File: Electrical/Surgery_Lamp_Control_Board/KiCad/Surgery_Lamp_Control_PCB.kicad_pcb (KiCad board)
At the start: 2 copper layers, 90 x 60 mm, 44 parts, among them J1 OSTVN05A150, J2 Headlamp, J3 Joint 1 Encoder, J4 Joint 2 Encoder, J5 joint2, J6 joint3, J7 joint4, J8 Stepper, Q1 BSS138, Q2 BSS138, Q3 BSS138, Q4 BSS138, Q5 BSS138, Q6 BSS138, U1 MAX485E, U2 PCA9685PW

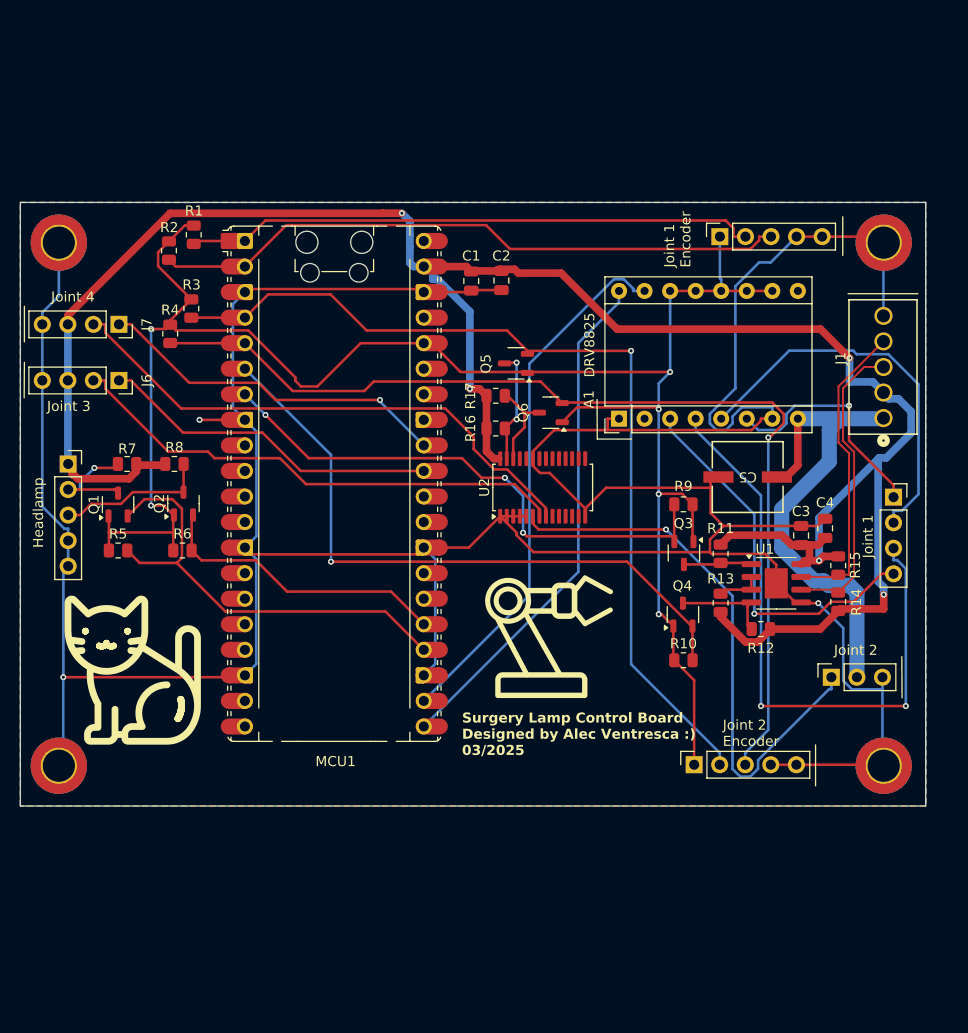
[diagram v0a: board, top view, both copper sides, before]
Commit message: Update Surgery Lamp Control PCB files
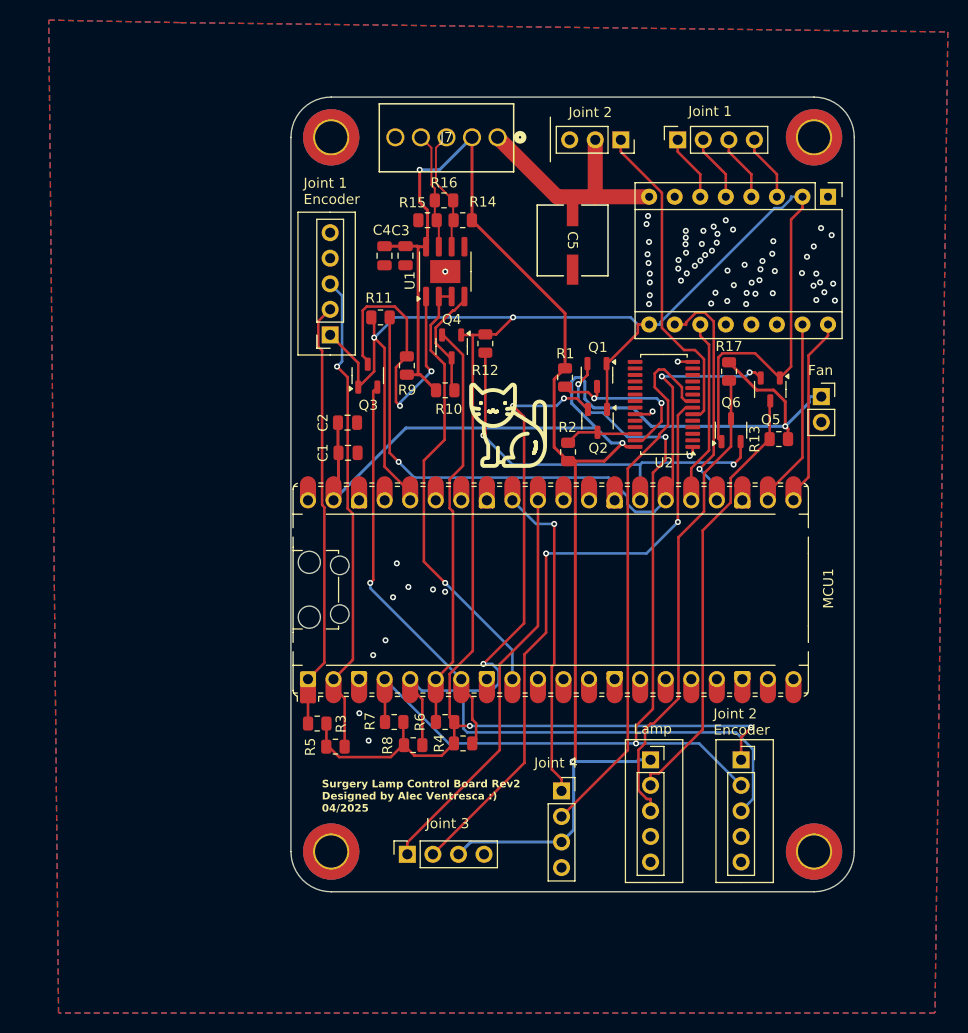
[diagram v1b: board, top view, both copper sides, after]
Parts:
- added J9: Fan, Connector_PinSocket_2.54mm:PinSocket_1x02_P2.54mm_Vertical, F.Cu at (176.0, 94.0)
- A1: value Pololu_Breakout_DRV8825 -> TMC2209 Stepper Driver
- J1: value OSTVN05A150 -> joint2; footprint Alec_lib:CONN5_516x256_OST -> Connector_PinSocket_2.54mm:PinSocket_1x03_P2.54mm_Vertical
- J2: value Headlamp -> joint3; footprint Connector_PinSocket_2.54mm:PinSocket_1x05_P2.54mm_Vertical -> Connector_PinSocket_2.54mm:PinSocket_1x04_P2.54mm_Vertical
- J3: value Joint 1 Encoder -> joint4; footprint Connector_PinSocket_2.54mm:PinSocket_1x05_P2.54mm_Vertical -> Connector_PinSocket_2.54mm:PinSocket_1x04_P2.54mm_Vertical
- J4: value Joint 2 Encoder -> Headlamp
- J5: value joint2 -> Joint 1 Encoder; footprint Connector_PinSocket_2.54mm:PinSocket_1x03_P2.54mm_Vertical -> Connector_PinSocket_2.54mm:PinSocket_1x05_P2.54mm_Vertical
- J6: value joint3 -> Joint 2 Encoder; footprint Connector_PinSocket_2.54mm:PinSocket_1x04_P2.54mm_Vertical -> Connector_PinSocket_2.54mm:PinSocket_1x05_P2.54mm_Vertical
- J7: value joint4 -> OSTVN05A150; footprint Connector_PinSocket_2.54mm:PinSocket_1x04_P2.54mm_Vertical -> Alec_lib:CONN5_516x256_OST
- R16: value 10k -> 120
- moved H3 96.4 mm to (175.2, 139.2)
- moved H4 81.7 mm to (127.2, 139.2)
- moved J6 72.4 mm to (168.0, 130.1), turned to 0 degrees
- moved H2 68.1 mm to (127.2, 68.2)
- moved H1 62.9 mm to (175.2, 68.2)
- moved J5 60.3 mm to (127.2, 87.9), turned to 180 degrees
- moved J3 57.3 mm to (150.2, 133.2), turned to 0 degrees
- moved R15 53.3 mm to (136.8, 76.5), turned to 180 degrees
- moved R14 53.2 mm to (140.3, 76.5), turned to 180 degrees
- moved C4 51.5 mm to (132.6, 80.0), turned to -90 degrees
- moved J2 51.4 mm to (134.8, 139.5), turned to 90 degrees
- moved R4 50.1 mm to (140.4, 128.5), turned to 0 degrees
- moved Q1 49.3 mm to (153.7, 91.9), turned to -90 degrees
- moved C3 48.2 mm to (134.6, 80.0), turned to -90 degrees
- moved U1 45.2 mm to (138.6, 81.6), turned to 90 degrees
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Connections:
- A1 pad 10: 3V3 -> MS1
- A1 pad 11: 3V3 -> MS2
- A1 pad 12: 3V3 -> unconnected-(A1-RX-Pad12)
- A1 pad 13: 3V3 -> unconnected-(A1-TX-Pad13)
- A1 pad 14: 3V3 -> unconnected-(A1-CLK-Pad14)
- A1 pad 2: unconnected-(A1-~{FLT}-Pad2) -> 3V3
- A1 pad 9: unconnected-(A1-~{EN}-Pad9) -> 3V3
- J1 pad 1: 24V -> Net-(J1-Pin_1)
- J1 pad 2: 5V -> 24V
- J1 pad 3: RS+ -> GND
- J2 pad 1: 5V -> joint3_Feedback
- J2 pad 2: neopixel -> Net-(J2-Pin_2)
- J2 pad 3: laser_pointer -> 5V
- J3 pad 1: 3V3 -> joint4_Feedback
- J3 pad 2: SDA0 -> Net-(J3-Pin_2)
- J3 pad 3: SCL0 -> 5V
- J4 pad 1: 3V3 -> 5V
- J4 pad 2: SDA1 -> neopixel
- J4 pad 3: SCL1 -> laser_pointer
- J5 pad 1: Net-(J5-Pin_1) -> 3V3
- J5 pad 2: 24V -> SDA0
- J5 pad 3: GND -> SCL0
- J6 pad 1: joint3_Feedback -> 3V3
- J6 pad 2: Net-(J6-Pin_2) -> SDA1
- J6 pad 3: 5V -> SCL1
- J7 pad 1: joint4_Feedback -> 24V
- J7 pad 2: Net-(J7-Pin_2) -> 5V
- J7 pad 3: 5V -> RS+
- J7 pad 4: GND -> RS-
- MCU1 pad 24: Net-(MCU1-GPIO18) -> MS1
- MCU1 pad 25: Net-(MCU1-GPIO19) -> MS2
- MCU1 pad 26: unconnected-(MCU1-GPIO20-Pad26)_1 -> Net-(MCU1-GPIO20)
- MCU1 pad 27: unconnected-(MCU1-GPIO21-Pad27)_1 -> Net-(MCU1-GPIO21)
- MCU1 pad 9: unconnected-(MCU1-GPIO6-Pad9)_1 -> RS_Enable
- Q1 pad 2: Net-(MCU1-GPIO18) -> SDA1
- Q1 pad 3: neopixel -> SDA1_5V
- Q2 pad 2: Net-(MCU1-GPIO19) -> SCL1
- Q2 pad 3: laser_pointer -> SCL1_5V
- Q5 pad 2: SDA1 -> Net-(MCU1-GPIO20)
- Q5 pad 3: SDA1_5V -> neopixel
- Q6 pad 2: SCL1 -> Net-(MCU1-GPIO21)
- Q6 pad 3: SCL1_5V -> laser_pointer
- R1 pad 1: 3V3 -> 5V
- R1 pad 2: SDA0 -> SDA1_5V
- R10 pad 1: 3V3 -> 5V
- R10 pad 2: TX -> Net-(Q4-D)
- R11 pad 1: 5V -> 3V3
- R11 pad 2: Net-(Q3-D) -> Net-(MCU1-GPIO20)
- R12 pad 1: 5V -> 3V3
- R12 pad 2: Net-(Q4-D) -> Net-(MCU1-GPIO21)
- R13 pad 2: Net-(U1-DE) -> neopixel
- R15 pad 1: 5V -> RS-
- R15 pad 2: RS- -> GND
- R16 pad 1: 5V -> RS+
- R16 pad 2: SDA1_5V -> RS-
- R17 pad 2: SCL1_5V -> laser_pointer
- R2 pad 1: 3V3 -> 5V
- R2 pad 2: SCL0 -> SCL1_5V
- R3 pad 2: SDA1 -> SDA0
- R4 pad 2: SCL1 -> RX
- R5 pad 2: Net-(MCU1-GPIO18) -> SCL0
- R6 pad 2: Net-(MCU1-GPIO19) -> TX
- R7 pad 1: 5V -> 3V3
- R7 pad 2: neopixel -> SDA1
- R8 pad 1: 5V -> 3V3
- R8 pad 2: laser_pointer -> SCL1
- R9 pad 1: 3V3 -> 5V
- R9 pad 2: RX -> Net-(Q3-D)
- U1 pad 2: Net-(U1-DE) -> RS_Enable
- U1 pad 3: Net-(U1-DE) -> RS_Enable
- U2 pad 6: Net-(J5-Pin_1) -> Net-(J1-Pin_1)
- U2 pad 7: Net-(J6-Pin_2) -> Net-(J2-Pin_2)
- U2 pad 8: Net-(J7-Pin_2) -> Net-(J3-Pin_2)
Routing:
- net GND: track 377.5 -> 4.37 mm, vias 3 -> 70
- net Net-(MCU1-GPIO20): track 0.00 -> 67.5 mm, vias 0 -> 3
- net Net-(J2-Pin_2): track 0.00 -> 61.4 mm, vias 0 -> 2
- net Net-(J5-Pin_1): track 56.2 -> 0.00 mm, vias 1 -> 0
- net Net-(A1-2A): track 62.1 -> 6.59 mm, vias 2 -> 0
- net Net-(J3-Pin_2): track 0.00 -> 54.8 mm
- net Net-(J7-Pin_2): track 54.5 -> 0.00 mm
- net Net-(J6-Pin_2): track 50.8 -> 0.00 mm
- net Net-(MCU1-GPIO18): track 46.4 -> 0.00 mm
- net RS_Enable: track 0.00 -> 45.5 mm, vias 0 -> 1
- net Net-(MCU1-GPIO21): track 0.00 -> 41.5 mm, vias 0 -> 2
- net 3V3: track 187.9 -> 227.0 mm, vias 6 -> 4
- net STEP: track 54.2 -> 18.9 mm
- net DIR: track 52.1 -> 18.9 mm
- net Net-(A1-1A): track 39.1 -> 6.59 mm
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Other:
- board size 90 x 60 mm -> 56 x 79 mm
- board text added: "Fan"
- board text added: "Lamp"
- board text added: "Surgery Lamp Control Board Rev2 Designed by Alec Ventresca :) 04/2025"
- board text removed: "DRV8825"
- board text removed: "Headlamp"
- board text removed: "Surgery Lamp Control Board Designed by Alec Ventresca :) 03/2025"
